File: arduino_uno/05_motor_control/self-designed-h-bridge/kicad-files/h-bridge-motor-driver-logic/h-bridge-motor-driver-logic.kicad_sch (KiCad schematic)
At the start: 9 parts, among them J1 Conn_01x04_Pin, J2 Conn_01x06_Pin, U1 PC847, U2 74HC14, U3 4011

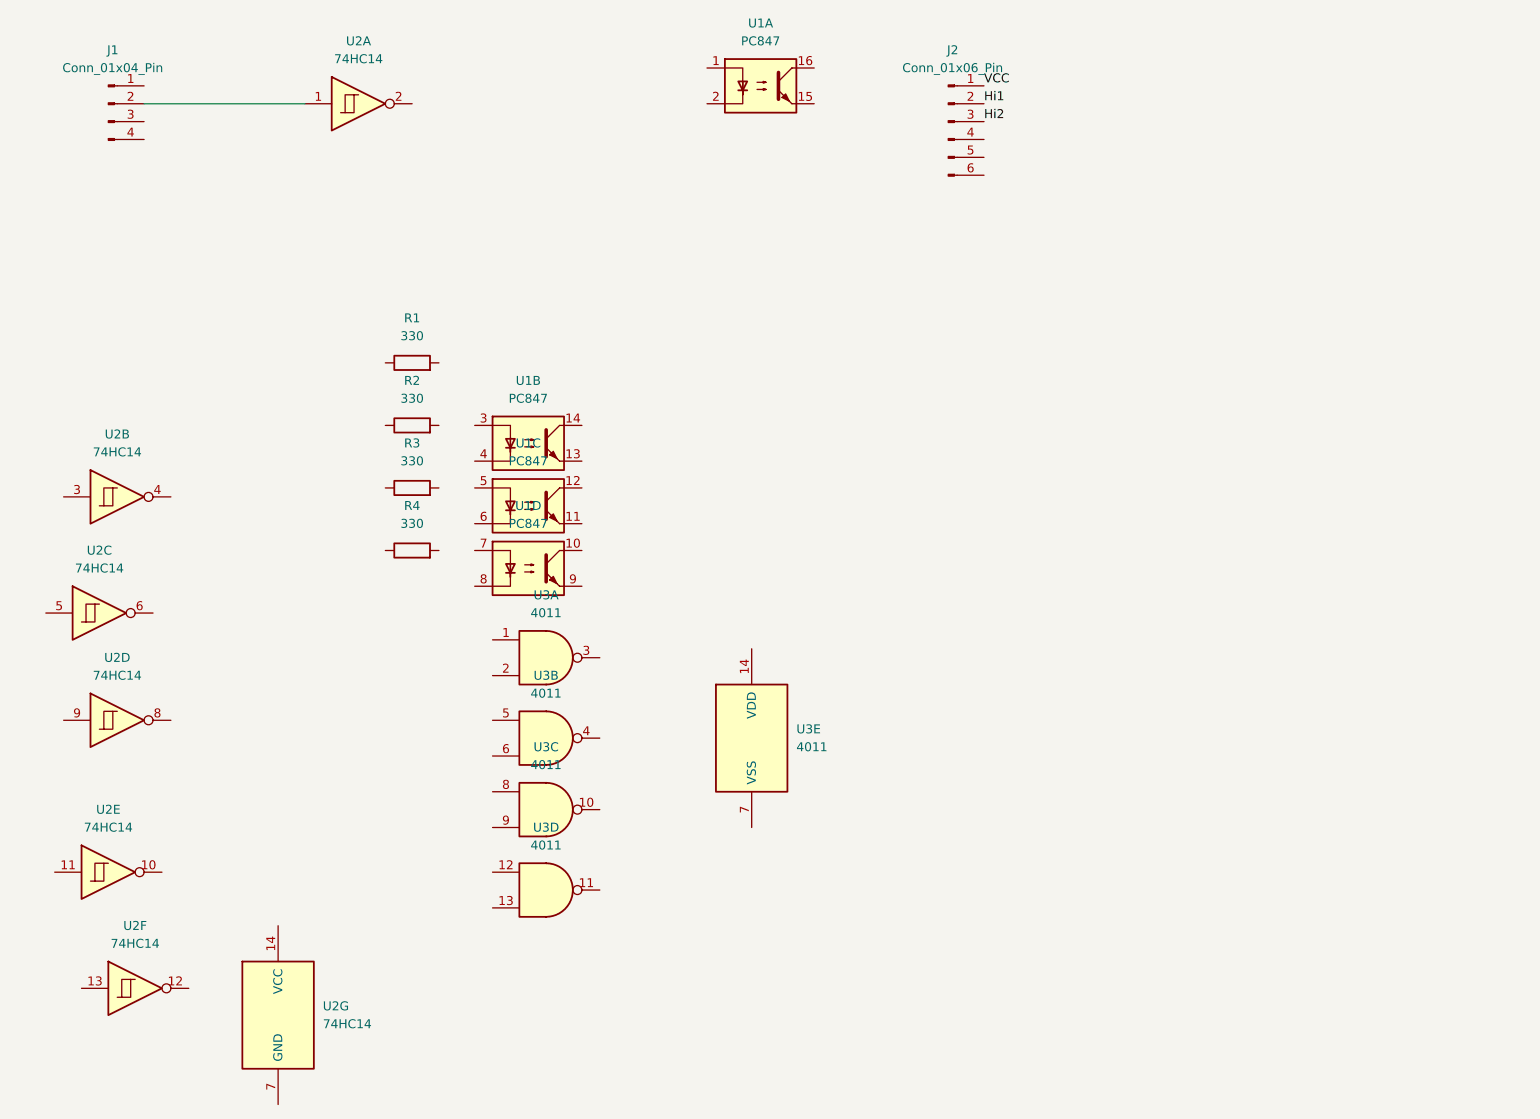
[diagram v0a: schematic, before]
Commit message: add wiring
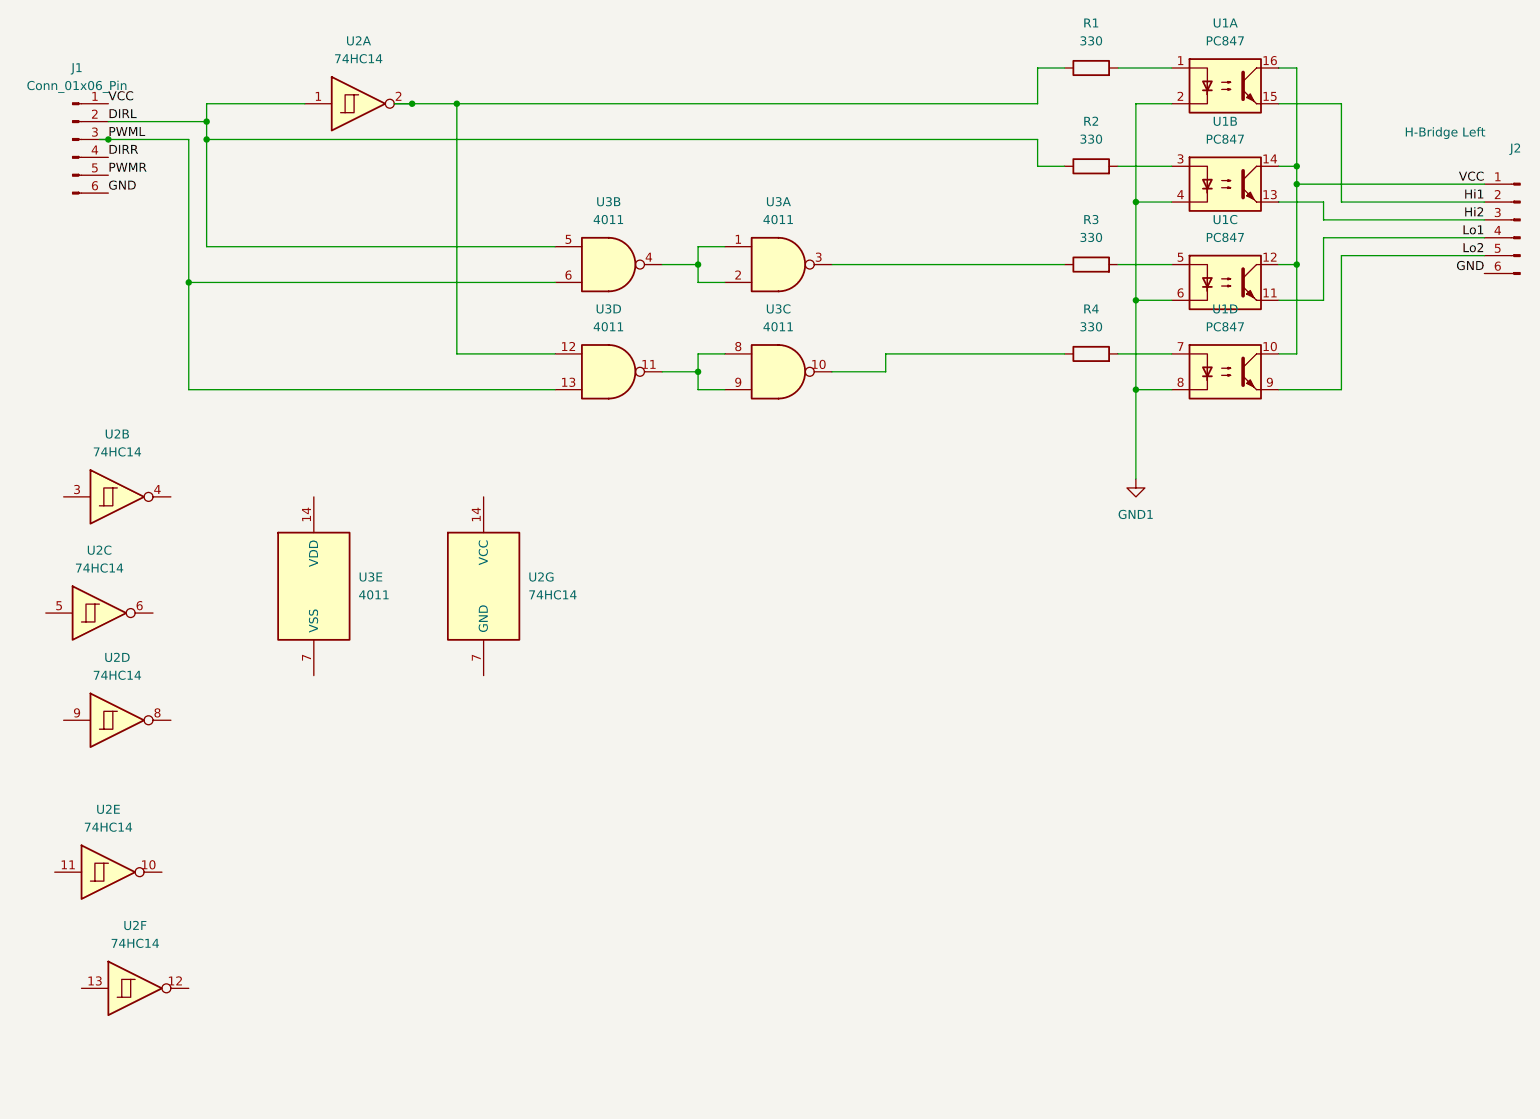
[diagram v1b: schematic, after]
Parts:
- removed J1: Conn_01x04_Pin, symbol Connector:Conn_01x04_Pin
- added J1: Conn_01x06_Pin, symbol Connector:Conn_01x06_Pin
- J2: value Conn_01x06_Pin -> H-Bridge Left
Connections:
- net Hi1: now also U1.15
- net Hi2: now also U1.13
- net VCC: now also U1.10, U1.12, U1.14, U1.16, J1.1 (Pin_1)
- net DIRL: now reaches R2.1
- net DIRL: now also U2.1, U3.5, J1.2 (Pin_2)
- net at R2.2: now also U1.3
- net at U1.7: now also R4.2
- net GND1: now reaches U1.8
- net GND1: now also U1.2, U1.4, U1.6
- net Lo2: now reaches U1.9
- net Lo2: now also J2.5 (Pin_5)
- net at R1.1: now also U2.2, U3.12
- net at R1.2: now also U1.1
- net at U3.11: now also U3.8, U3.9
- net PWML: now reaches U3.13
- net PWML: now also U3.6, J1.3 (Pin_3)
- net Lo1: now reaches J2.4 (Pin_4)
- net Lo1: now also U1.11
- net GND: now reaches J2.6 (Pin_6)
- net GND: now also J1.6 (Pin_6)
- net at U3.10: now also R4.1
- net at U3.1: now also U3.2, U3.4
- net at U3.3: now also R3.1
- net at U1.5: now also R3.2
- new net DIRR: J1.4 (Pin_4)
- new net PWMR: J1.5 (Pin_5)
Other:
- moved on the sheet: J2, R1, R2, R3, R4, U1A, U1B, U1C, U1D, U2G, U3A, U3B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
